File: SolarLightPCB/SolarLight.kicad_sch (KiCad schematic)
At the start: 19 parts, among them J1 I2C, J2 SPI, SW1 RotaryEncoder_Switch, U1 TP4056, U2 WeMos_D1_mini, U3 MCP1700-3302E

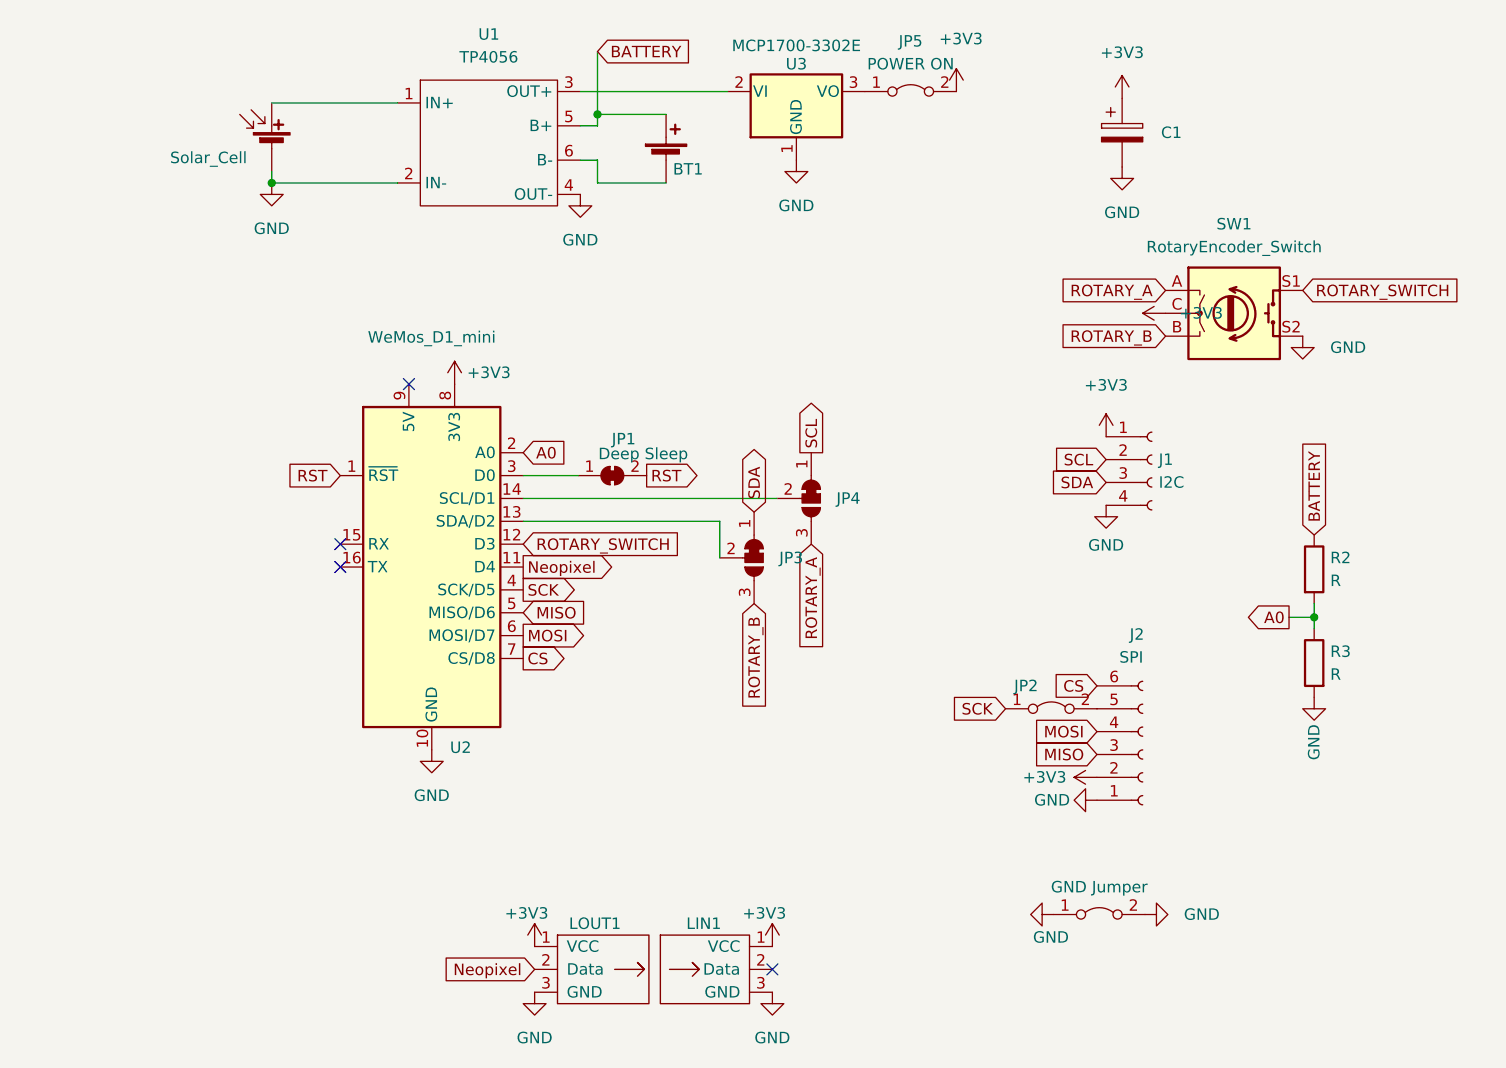
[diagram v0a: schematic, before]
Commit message: Make a “simplified” version
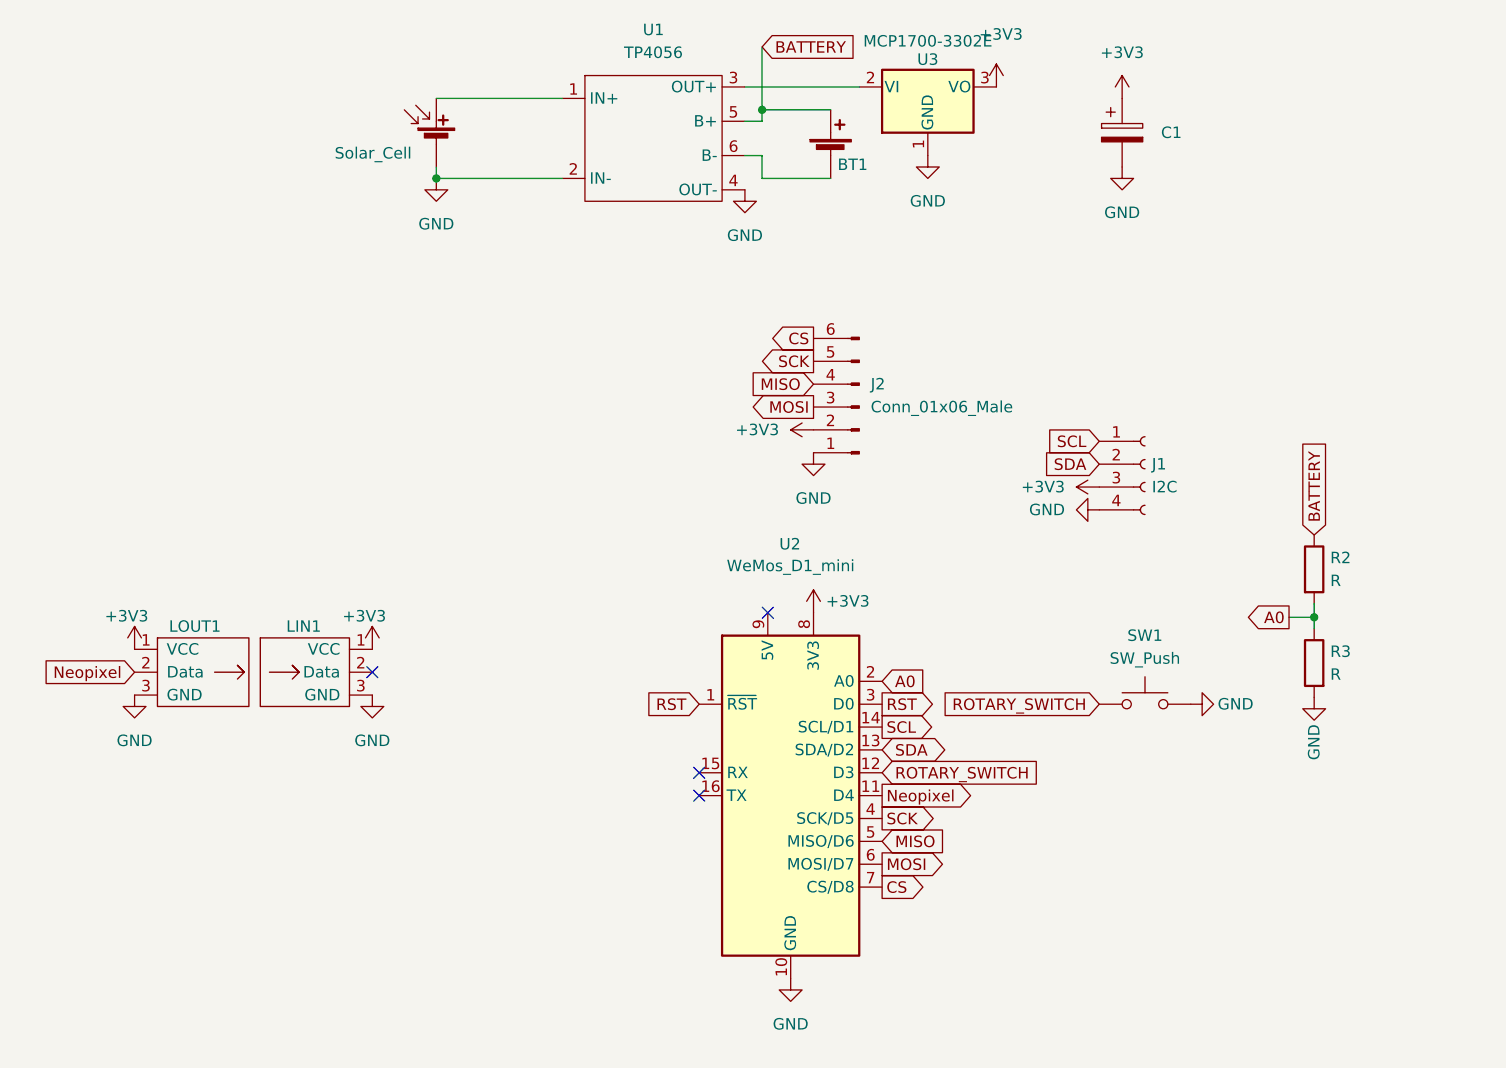
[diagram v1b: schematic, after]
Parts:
- removed J2: SPI, Connector_PinHeader_2.54mm:PinHeader_1x06_P2.54mm_Vertical, symbol Connector:Conn_01x06_Female
- removed JP1: Deep Sleep, Jumper:SolderJumper-2_P1.3mm_Bridged_Pad1.0x1.5mm, symbol Jumper:SolderJumper_2_Bridged
- removed JP2: Jumper_2_Bridged, Resistor_THT:R_Axial_DIN0204_L3.6mm_D1.6mm_P5.08mm_Horizontal, symbol Jumper:Jumper_2_Bridged
- removed JP3, JP4: SolderJumper_3_Bridged12, Jumper:SolderJumper-3_P1.3mm_Bridged12_Pad1.0x1.5mm, symbol Jumper:SolderJumper_3_Bridged12
- removed JP5: POWER ON, Connector_PinHeader_2.54mm:PinHeader_1x02_P2.54mm_Vertical, symbol Jumper:Jumper_2_Bridged
- removed JP6: GND Jumper, Resistor_THT:R_Axial_DIN0204_L3.6mm_D1.6mm_P5.08mm_Horizontal, symbol Jumper:Jumper_2_Bridged
- removed SW1: RotaryEncoder_Switch, Rotary_Encoder:RotaryEncoder_Alps_EC12E-Switch_Vertical_H20mm, symbol Device:RotaryEncoder_Switch
- added J2: Conn_01x06_Male, Connector_PinHeader_2.54mm:PinHeader_1x06_P2.54mm_Vertical, symbol Connector:Conn_01x06_Male
- added SW1: SW_Push, Button_Switch_THT:SW_PUSH_6mm_H4.3mm, symbol Switch:SW_Push
- BT1, SC1: footprint Connector_PinHeader_2.54mm:PinHeader_1x02_P2.54mm_Vertical -> TerminalBlock_Phoenix:TerminalBlock_Phoenix_PT-1,5-2-3.5-H_1x02_P3.50mm_Horizontal
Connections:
- net +3V3: now also J1.3 (Pin_3), U3.3 (VO), J2.2 (Pin_2); no longer J1.1 (Pin_1)
- net CS: now also J2.6 (Pin_6)
- net GND: now also J2.1 (Pin_1), SW1.2
- net MISO: now also J2.4 (Pin_4)
- net MOSI: now also J2.3 (Pin_3)
- net ROTARY_SWITCH: now also SW1.1
- net RST: now also U2.3 (D0)
- net SCK: now also J2.5 (Pin_5)
- net SCL: now also J1.1 (Pin_1), U2.14 (SCL/D1); no longer J1.2 (Pin_2)
- net SDA: now also J1.2 (Pin_2), U2.13 (SDA/D2); no longer J1.3 (Pin_3)
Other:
- moved on the sheet: BT1, J1, LIN1, LOUT1, U1, U2, U3
